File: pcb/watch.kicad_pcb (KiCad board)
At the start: 6 copper layers, 47.2 x 35.5 mm, 61 parts, among them J1 USB_C_Receptacle_USB2.0_14P, J2 Adafruit Wireless Chg Module, U1 nRF52840, U2 USBLC6-2SC6, U3 MAX-M10S, U4 TPS63802DLAR, U5 TPS7A20xxxDQN, U6 BQ24074RGT, U8 RV-3028-C7, U9 TPS2116DRL, Y1 32MHz

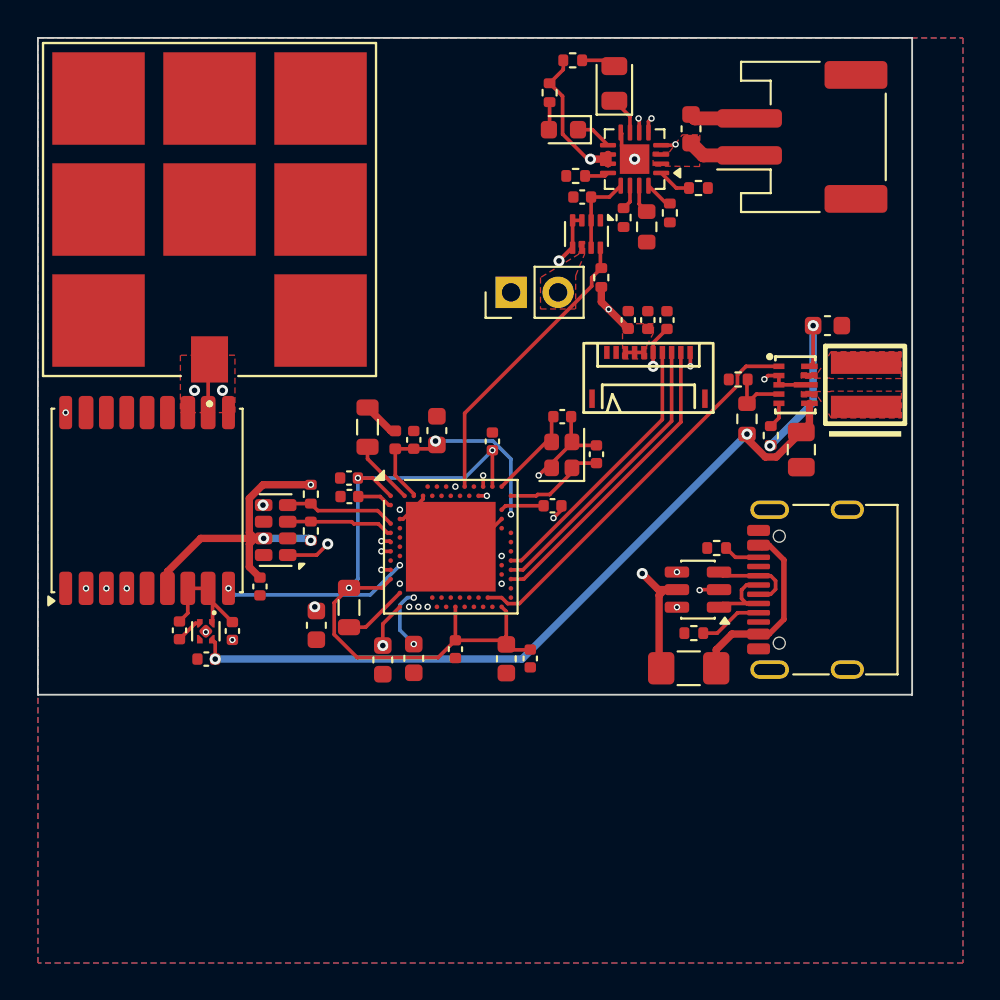
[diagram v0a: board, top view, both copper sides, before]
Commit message: almost done?
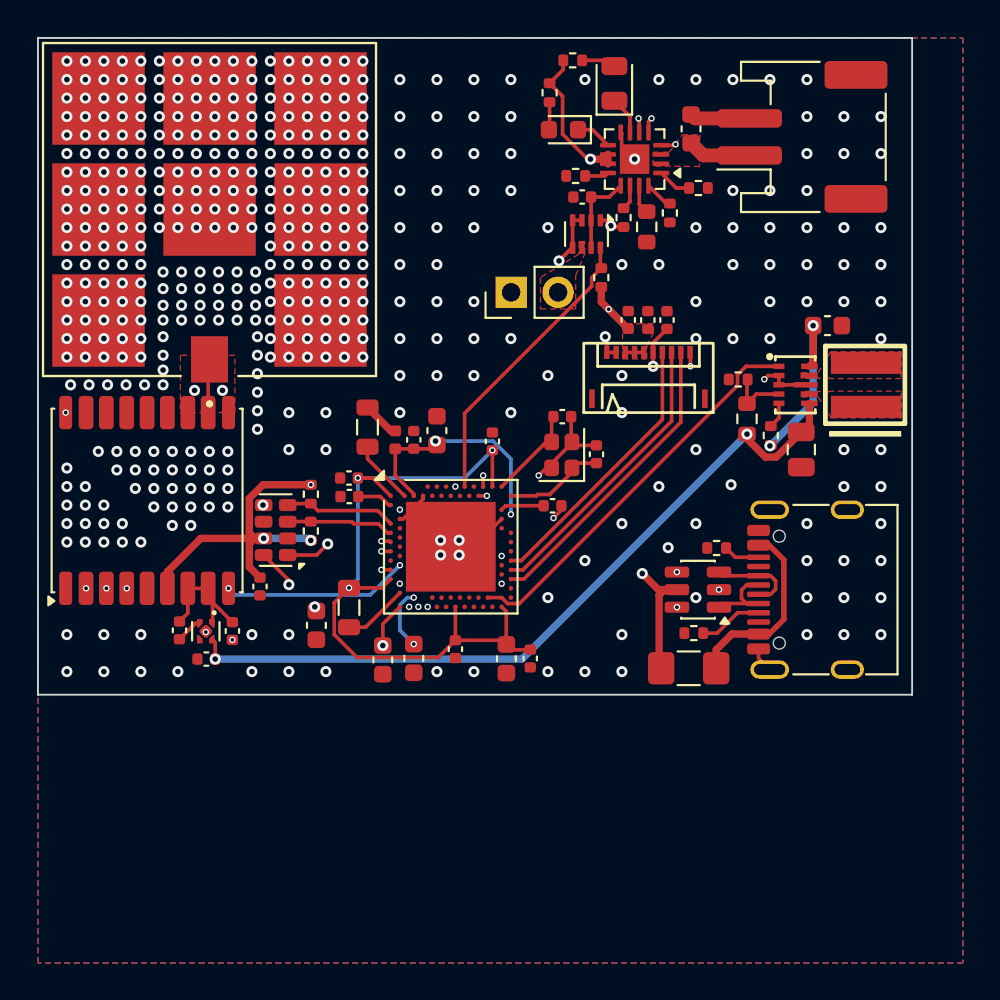
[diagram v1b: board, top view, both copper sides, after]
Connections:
- E1 pad 2: (no net) -> GND
- E1 pad 3: (no net) -> GND
- E1 pad 4: (no net) -> GND
- E1 pad 5: (no net) -> GND
- E1 pad 6: (no net) -> GND
- E1 pad 7: (no net) -> GND
- E1 pad 8: (no net) -> GND
- E1 pad 9: (no net) -> GND
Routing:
- net GND: track 22.0 -> 27.2 mm, vias 8 -> 464
- net Net-(U3-RF_IN): track 3.66 -> 2.91 mm
